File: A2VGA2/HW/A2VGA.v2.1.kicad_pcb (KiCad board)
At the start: 2 copper layers, 65.5 x 79.8 mm, 66 parts, among them U1 CPB

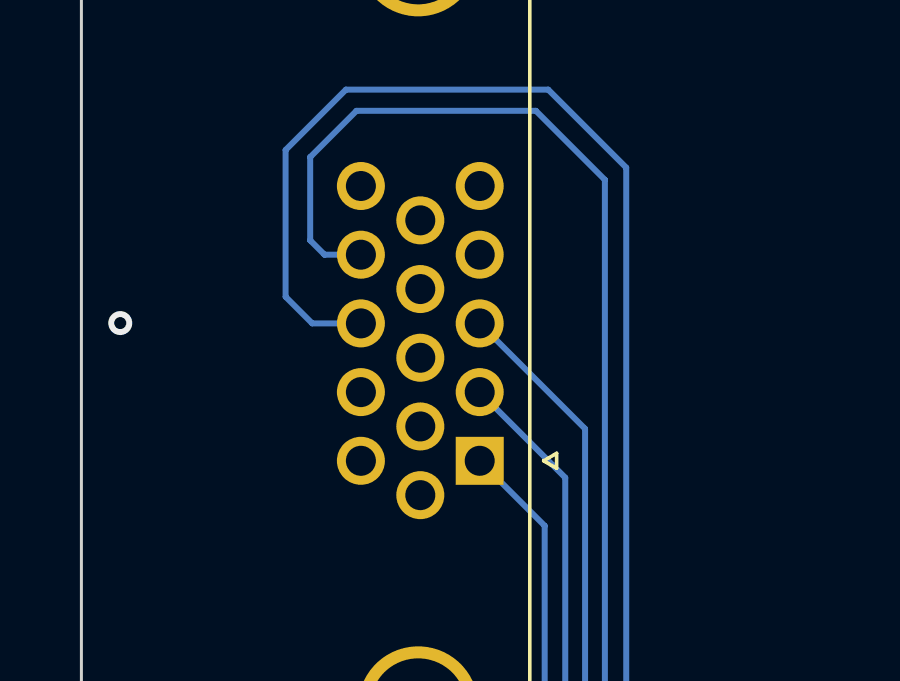
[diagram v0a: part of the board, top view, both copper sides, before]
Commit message: Add files via upload
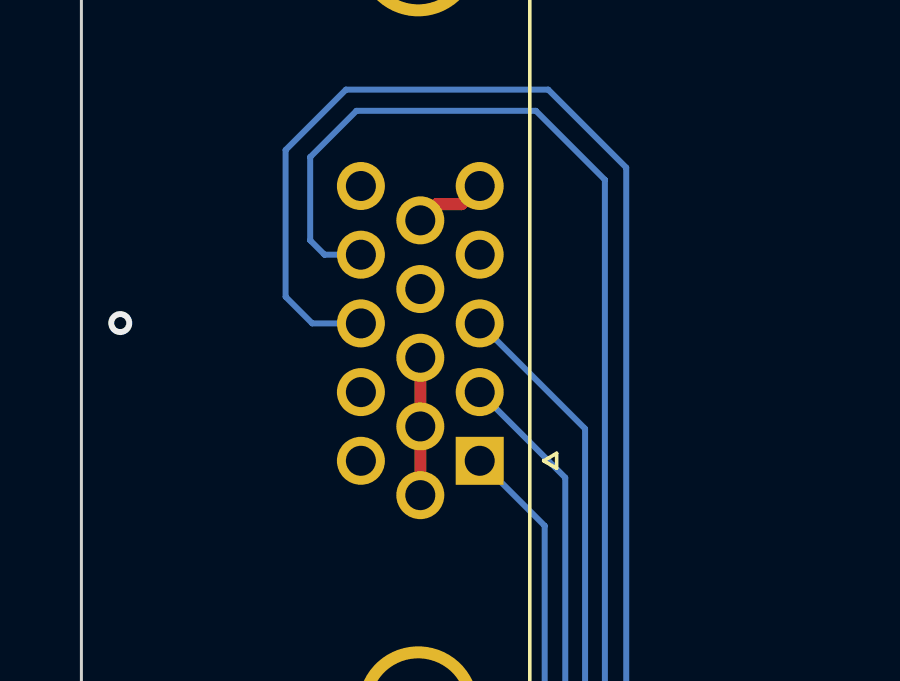
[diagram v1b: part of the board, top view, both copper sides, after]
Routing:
- net GND: track 4.95 -> 12.0 mm
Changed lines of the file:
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@@
 		(net 0)
+	)
+	(segment
+		(start 163.1114 70.4628)
+		(end 162.505 71.0692)
+		(width 0.4)
+		(layer "F.Cu")
+		(net 1)
+	)
+	(segment
+		(start 161.1314 78.4778)
+		(end 161.1314 80.7678)
+		(width 0.4)
+		(layer "F.Cu")
+		(net 1)
+	)
+	(segment
+		(start 162.505 71.0692)
+		(end 161.67 71.0692)
+		(width 0.4)
+		(layer "F.Cu")
+		(net 1)
+	)
+	(segment
+		(start 161.1314 78.4778)
+		(end 161.1314 76.1878)
+		(width 0.4)
+		(layer "F.Cu")
+		(net 1)
+	)
+	(segment
+		(start 161.67 71.0692)
+		(end 161.1314 71.6078)
+		(width 0.4)
+		(layer "F.Cu")
+		(net 1)
 	)
 	(via
